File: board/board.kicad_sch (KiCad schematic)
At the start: 2 parts

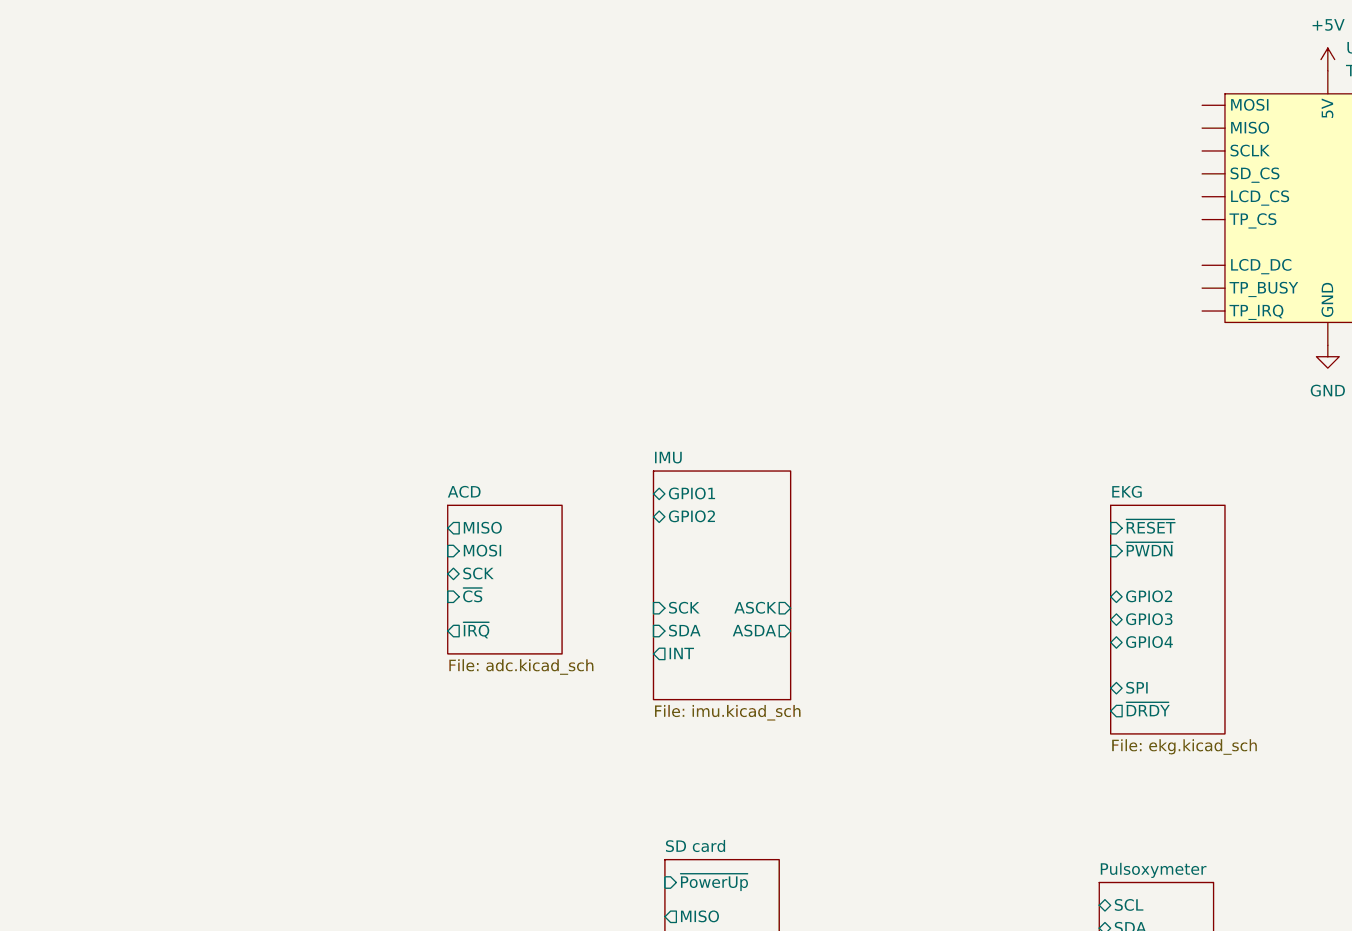
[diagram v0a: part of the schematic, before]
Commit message: updated schematic after review
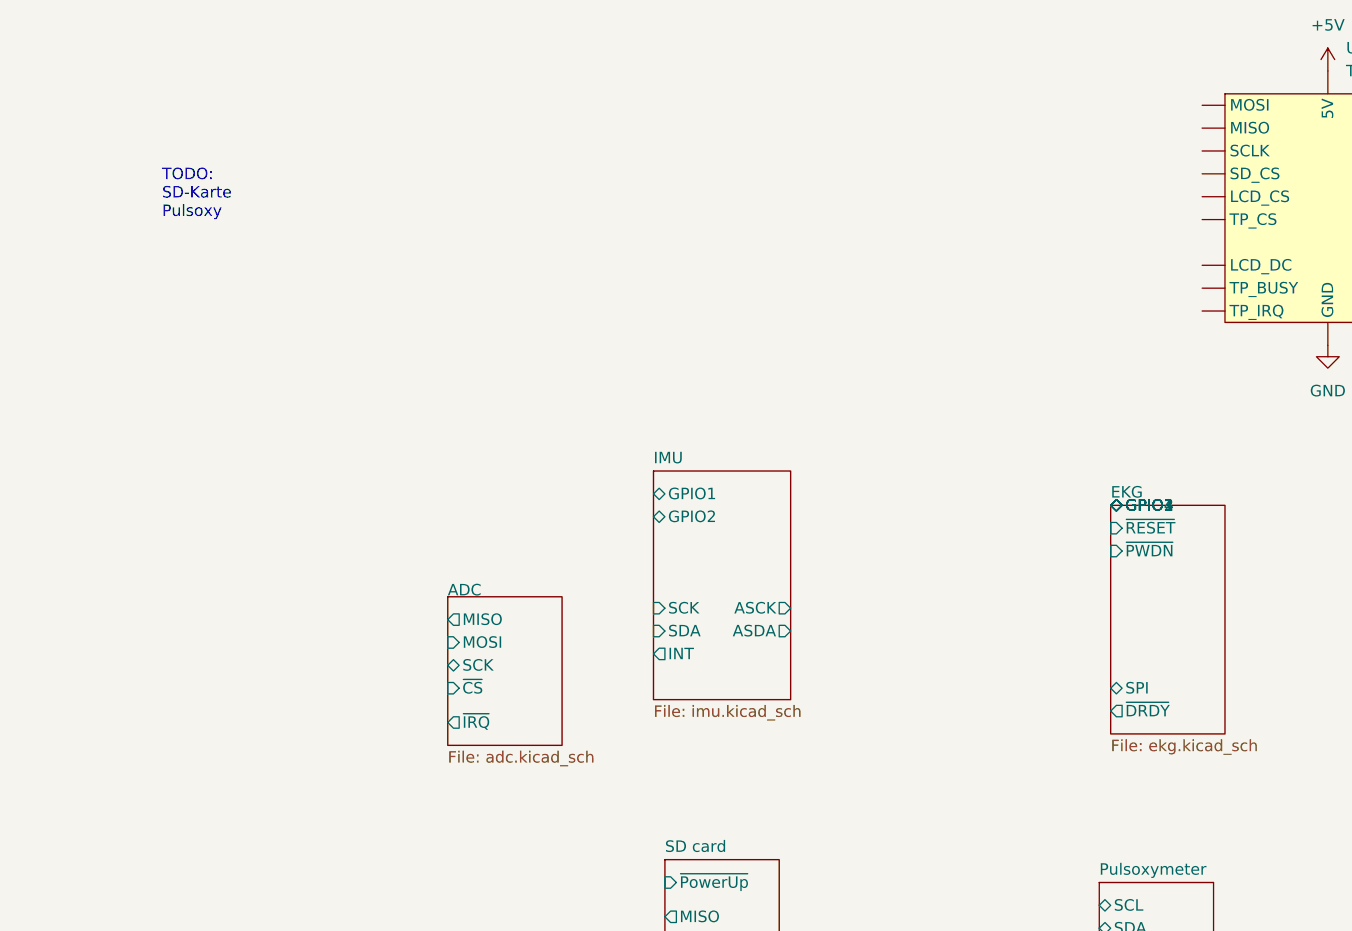
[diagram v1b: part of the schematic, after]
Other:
- sheet ACD renamed ADC
- sheet EKG ports: added GPIO1; removed none
- note added: "TODO: SD-Karte Pulsoxy"
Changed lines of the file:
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@@
 (kicad_sch (version 20211123) (generator eeschema)
   (paper "A4")
+  (text "TODO:\nSD-Karte\nPulsoxy" (at 109.22 62.23 0)
+    (effects (font (size 1.27 1.27)) (justify left bottom))
+  )
   (symbol (lib_id "ownLib:TFT_Touch_Shield_WaveShare") (at 238.76 59.69 0) (unit 1)
     (in_bom yes) (on_board yes) (fields_autoplaced)
@@
     )
   )
-  (sheet (at 140.97 93.98) (size 12.7 16.51) (fields_autoplaced)
-    (stroke (width 0.1524) (type solid) (color 0 0 0 0))
-    (fill (color 0 0 0 0.0000))
-    (property "Sheet name" "ACD" (id 0) (at 140.97 93.2684 0)
-      (effects (font (size 1.27 1.27)) (justify left bottom))
-    )
-    (property "Sheet file" "adc.kicad_sch" (id 1) (at 140.97 111.0746 0)
-      (effects (font (size 1.27 1.27)) (justify left top))
-    )
-    (pin "MOSI" input (at 140.97 99.06 180)
-      (effects (font (size 1.27 1.27)) (justify left))
-    )
-    (pin "MISO" output (at 140.97 96.52 180)
-      (effects (font (size 1.27 1.27)) (justify left))
-    )
-    (pin "SCK" bidirectional (at 140.97 101.6 180)
-      (effects (font (size 1.27 1.27)) (justify left))
-    )
-    (pin "~{CS}" input (at 140.97 104.14 180)
-      (effects (font (size 1.27 1.27)) (justify left))
-    )
-    (pin "~{IRQ}" output (at 140.97 107.95 180)
+  (sheet (at 140.97 104.14) (size 12.7 16.51)
+    (stroke (width 0.1524) (type solid) (color 0 0 0 0))
+    (fill (color 0 0 0 0.0000))
+    (property "Sheet name" "ADC" (id 0) (at 140.97 104.14 0)
+      (effects (font (size 1.27 1.27)) (justify left bottom))
+    )
+    (property "Sheet file" "adc.kicad_sch" (id 1) (at 140.97 121.2346 0)
+      (effects (font (size 1.27 1.27)) (justify left top))
+    )
+    (pin "MOSI" input (at 140.97 109.22 180)
+      (effects (font (size 1.27 1.27)) (justify left))
+    )
+    (pin "MISO" output (at 140.97 106.68 180)
+      (effects (font (size 1.27 1.27)) (justify left))
+    )
+    (pin "SCK" bidirectional (at 140.97 111.76 180)
+      (effects (font (size 1.27 1.27)) (justify left))
+    )
+    (pin "~{CS}" input (at 140.97 114.3 180)
+      (effects (font (size 1.27 1.27)) (justify left))
+    )
+    (pin "~{IRQ}" output (at 140.97 118.11 180)
       (effects (font (size 1.27 1.27)) (justify left))
     )
@@
       (effects (font (size 1.27 1.27)) (justify left))
     )
-    (pin "GPIO4" bidirectional (at 214.63 109.22 180)
-      (effects (font (size 1.27 1.27)) (justify left))
-    )
-    (pin "GPIO3" bidirectional (at 214.63 106.68 180)
-      (effects (font (size 1.27 1.27)) (justify left))
-    )
-    (pin "GPIO2" bidirectional (at 214.63 104.14 180)
+    (pin "GPIO4" bidirectional (at 214.63 93.98 180)
+      (effects (font (size 1.27 1.27)) (justify left))
+    )
+    (pin "GPIO3" bidirectional (at 214.63 93.98 180)
+      (effects (font (size 1.27 1.27)) (justify left))
+    )
+    (pin "GPIO2" bidirectional (at 214.63 93.98 180)
       (effects (font (size 1.27 1.27)) (justify left))
     )
@@
     )
     (pin "~{PWDN}" input (at 214.63 99.06 180)
+      (effects (font (size 1.27 1.27)) (justify left))
+    )
+    (pin "GPIO1" bidirectional (at 214.63 93.98 180)
       (effects (font (size 1.27 1.27)) (justify left))
     )
@@
       (reference "#PWR?") (unit 1) (value "+3.3VA") (footprint "")
     )
+    (path "/db6b8362-1493-4107-af7d-a8faca8bb053/5b87a2ce-4929-417b-95fa-cd030e59a5ec"
+      (reference "#PWR?") (unit 1) (value "+3V3") (footprint "")
+    )
     (path "/0133fba6-5aa6-4171-8a60-95549c0db33b/5ba70fc5-860b-413d-b200-2c0dbf8bb502"

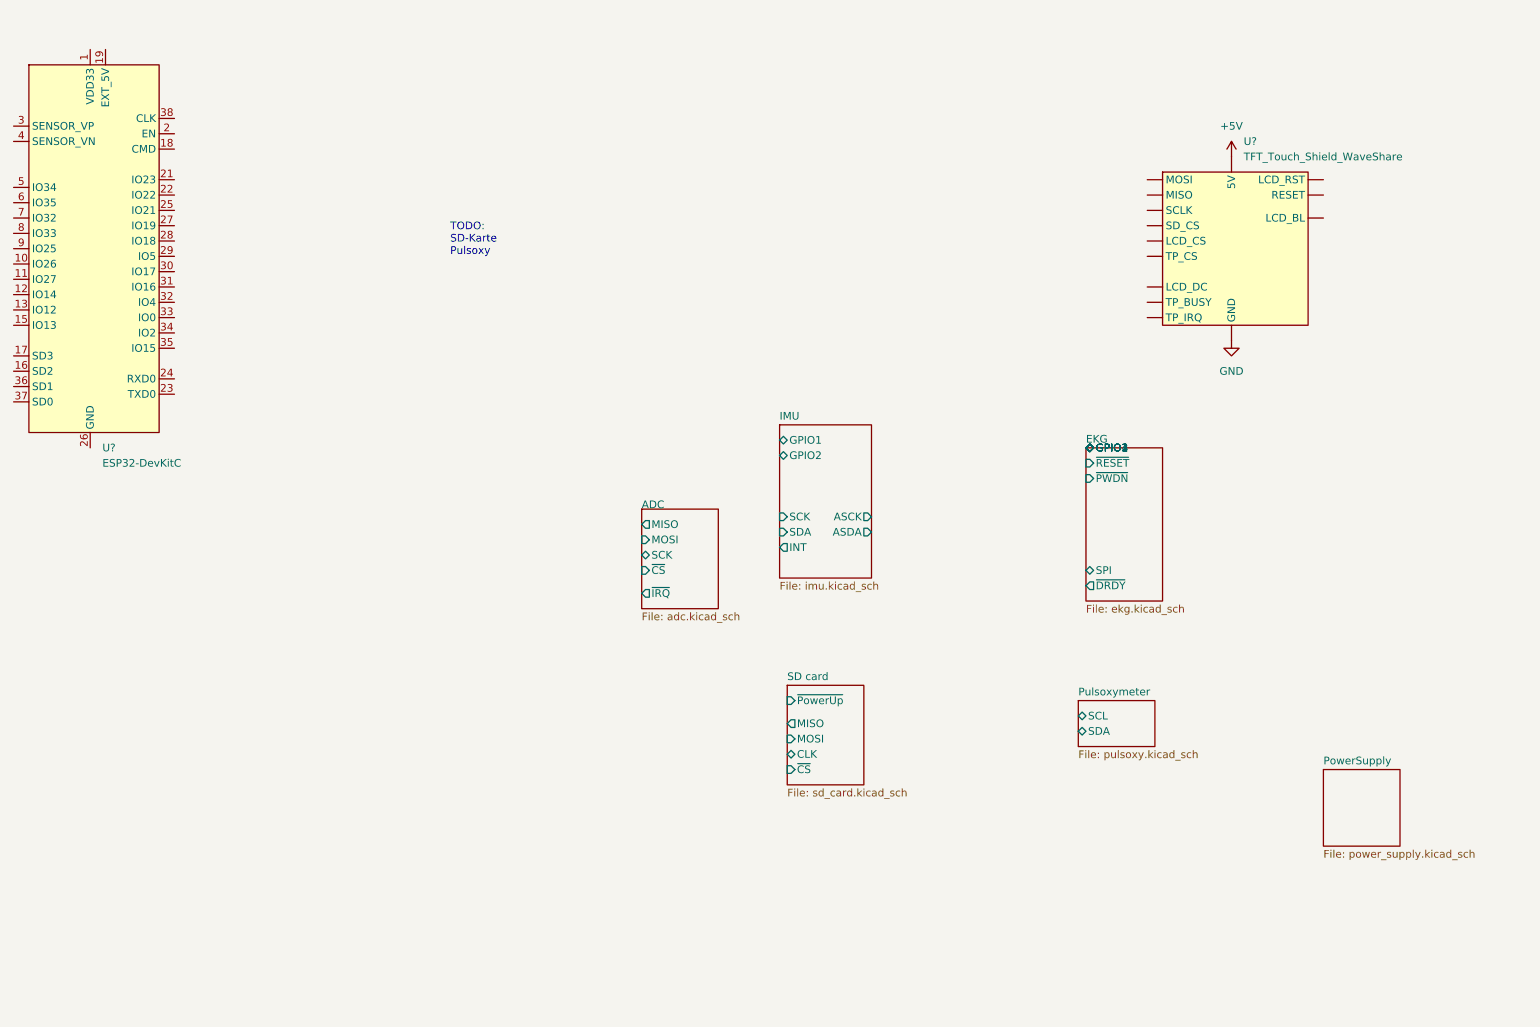
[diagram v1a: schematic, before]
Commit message: updated schematic
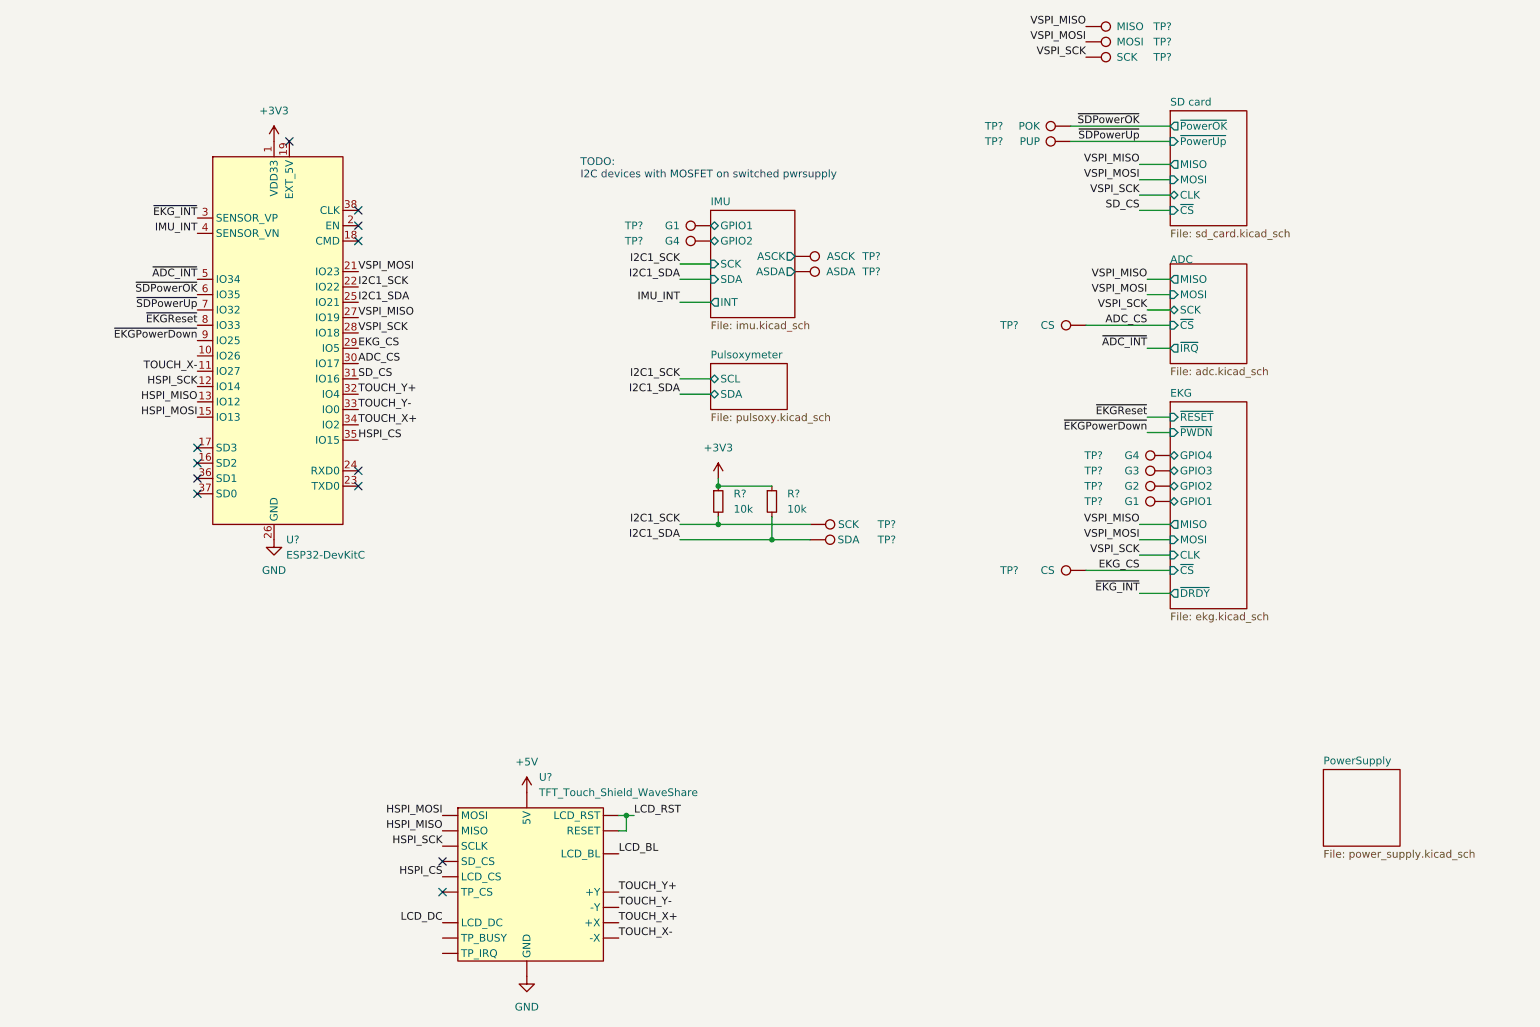
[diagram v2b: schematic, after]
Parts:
- added R? (x2): 10k, symbol Device:R_Small
- added TP?: ASCK, symbol Connector:TestPoint
- added TP? (x2): G1, symbol Connector:TestPoint
- added TP? (x2): G4, symbol Connector:TestPoint
- added TP?: G2, symbol Connector:TestPoint
- added TP?: ASDA, symbol Connector:TestPoint
- added TP?: MOSI, symbol Connector:TestPoint
- added TP?: PUP, symbol Connector:TestPoint
- added TP? (x2): CS, symbol Connector:TestPoint
- added TP?: MISO, symbol Connector:TestPoint
- added TP?: POK, symbol Connector:TestPoint
- added TP? (x2): SCK, symbol Connector:TestPoint
- added TP?: SDA, symbol Connector:TestPoint
- added TP?: G3, symbol Connector:TestPoint
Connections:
- net EKG/GPIO1: now also TP?.1
- net IMU/ASCK: now also TP?.1
- net IMU/ASDA: now also TP?.1
- net IMU/GPIO1: now also TP?.1
- net IMU/GPIO2: now also TP?.1
- net TOUCH_Y-: now reaches U?. (SCLK)
- net TOUCH_Y-: now also U?.33 (IO0)
- net +3V3: now reaches U?.1 (VDD33)
- net +3V3: now also R?.1, R?.1
- net TOUCH_X-: now reaches U?.11 (IO27)
- net TOUCH_X-: now also U?. (SCLK)
- net HSPI_SCK: now reaches U?.12 (IO14)
- net HSPI_SCK: now also U?. (SCLK)
- net HSPI_MISO: now reaches U?.13 (IO12)
- net HSPI_MISO: now also U?. (SCLK)
- net HSPI_MOSI: now reaches U?.15 (IO13)
- net HSPI_MOSI: now also U?. (SCLK)
- net VSPI_MOSI: now reaches U?.21 (IO23)
- net VSPI_MOSI: now also TP?.1
- net I2C1_SCK: now reaches U?.22 (IO22)
- net I2C1_SCK: now also R?.2, TP?.1
- net I2C1_SDA: now reaches U?.25 (IO21)
- net I2C1_SDA: now also R?.2, TP?.1
- net VSPI_MISO: now reaches U?.27 (IO19)
- net VSPI_MISO: now also TP?.1
- net VSPI_SCK: now reaches U?.28 (IO18)
- net VSPI_SCK: now also TP?.1
- net EKG_CS: now reaches U?.29 (IO5)
- net EKG_CS: now also TP?.1
- net ~{EKG_INT}: now reaches U?.3 (SENSOR_VP)
- net ADC_CS: now reaches U?.30 (IO17)
- net ADC_CS: now also TP?.1
- net SD_CS: now reaches U?.31 (IO16)
- net TOUCH_Y+: now reaches U?.32 (IO4)
- net TOUCH_Y+: now also U?. (SCLK)
- net TOUCH_X+: now reaches U?.34 (IO2)
- net TOUCH_X+: now also U?. (SCLK)
- net HSPI_CS: now reaches U?.35 (IO15)
- net HSPI_CS: now also U?. (SCLK)
- net IMU_INT: now reaches U?.4 (SENSOR_VN)
- net ~{ADC_INT}: now reaches U?.5 (IO34)
- net ~{SDPowerOK}: now reaches U?.6 (IO35)
- net ~{SDPowerOK}: now also TP?.1
- net ~{SDPowerUp}: now reaches U?.7 (IO32)
- net ~{SDPowerUp}: now also TP?.1
- net ~{EKGReset}: now reaches U?.8 (IO33)
- net ~{EKGPowerDown}: now reaches U?.9 (IO25)
- new net EKG/GPIO2: TP?.1
- new net EKG/GPIO3: TP?.1
- new net EKG/GPIO4: TP?.1
- new net LCD_BL: U?. (SCLK)
- new net LCD_DC: U?. (SCLK)
- new net LCD_RST: U?. (SCLK)
- no-connect marks 0 -> 12
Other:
- sheet EKG ports: added CLK, MISO, MOSI, ~{CS}; removed SPI
- sheet SD card ports: added ~{PowerOK}; removed none
- note added: "TODO: I2C devices with MOSFET on switched pwrsupply"
- note removed: "TODO: SD-Karte Pulsoxy"
- moved on the sheet: U?
